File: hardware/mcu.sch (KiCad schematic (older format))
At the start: 57 parts, among them P3 CONN_01X09, P4 CONN_02X05_JTAG, P5 CONN_01X03_UART, P6 CONN_01X03_CAN, P7 CONN_01X05_ENCODER, SW2 SW_PUSH, U13 TM4C1294KCPDT, U14 74LVCH2T45, U15 SN65HVD231D, Y1 NX5032GA

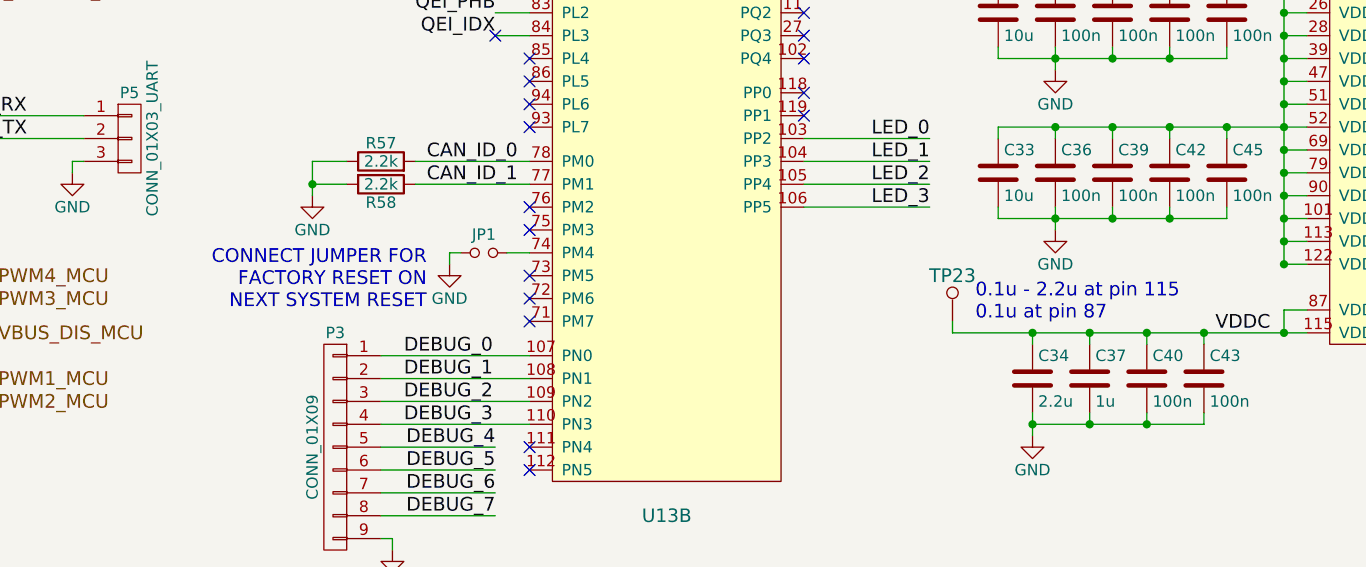
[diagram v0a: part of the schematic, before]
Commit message: tweaks, testpoints, decluttering
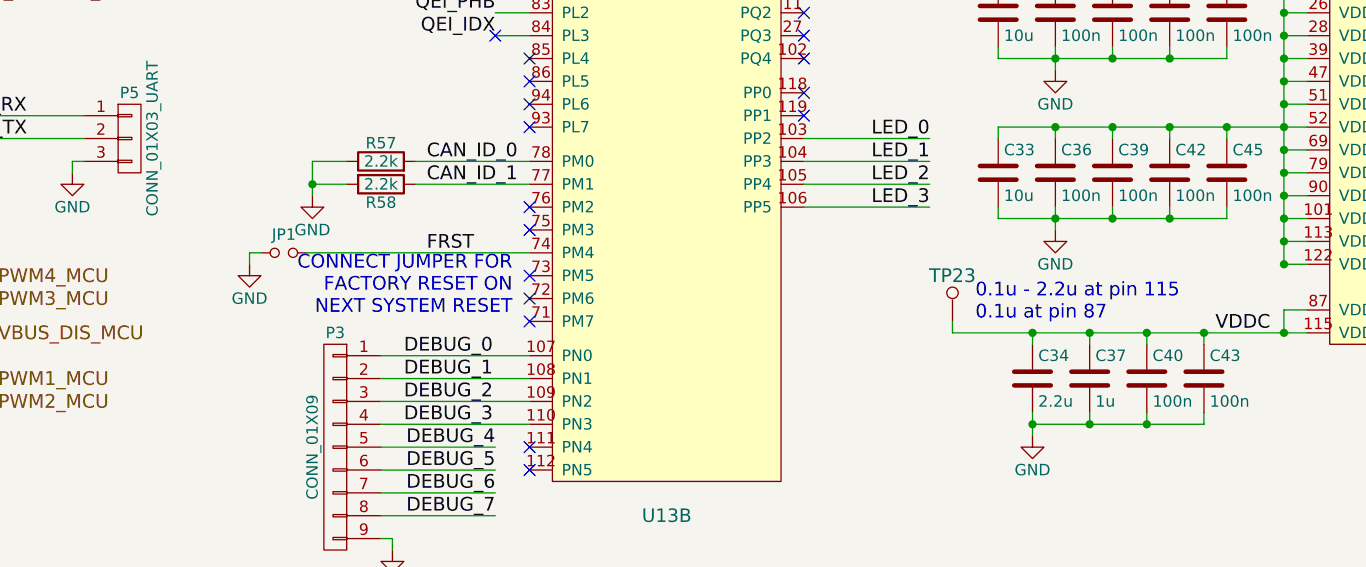
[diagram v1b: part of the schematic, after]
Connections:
- net FRST: now reaches JP1.1, U13.74 (PM4)
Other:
- moved on the sheet: JP1
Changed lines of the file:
@@
 L Jumper_NO_Small JP1
 U 1 1 59C1D74D
-P 5850 2300
-F 0 "JP1" H 5850 2380 50  0000 C CNN
-F 1 "Jumper_NO_Small" H 5860 2240 50  0001 C CNN
-F 2 "Pin_Headers:Pin_Header_Straight_1x02" H 5850 2300 50  0001 C CNN
-F 3 "" H 5850 2300 50  0000 C CNN
-	1    5850 2300
+P 4975 2300
+F 0 "JP1" H 4975 2380 50  0000 C CNN
+F 1 "Jumper_NO_Small" H 4985 2240 50  0001 C CNN
+F 2 "Pin_Headers:Pin_Header_Straight_1x02" H 4975 2300 50  0001 C CNN
+F 3 "" H 4975 2300 50  0000 C CNN
+	1    4975 2300
 	-1   0    0    -1
 $EndComp
@@
 L GND #PWR091
 U 1 1 59C1E162
-P 5700 2350
-F 0 "#PWR091" H 5700 2100 50  0001 C CNN
-F 1 "GND" H 5700 2200 50  0000 C CNN
-F 2 "" H 5700 2350 50  0000 C CNN
-F 3 "" H 5700 2350 50  0000 C CNN
-	1    5700 2350
+P 4825 2350
+F 0 "#PWR091" H 4825 2100 50  0001 C CNN
+F 1 "GND" H 4825 2200 50  0000 C CNN
+F 2 "" H 4825 2350 50  0000 C CNN
+F 3 "" H 4825 2350 50  0000 C CNN
+	1    4825 2350
 	-1   0    0    -1
 $EndComp
-Text Notes 5600 2550 2    60   ~ 0
+Text Notes 5975 2575 2    60   ~ 0
 CONNECT JUMPER FOR\nFACTORY RESET ON\nNEXT SYSTEM RESET
 $Comp
@@
 	8250 2700 8250 2650
 Wire Wire Line
-	8500 2700 8500 2650
+	8500 2650 8500 2700
 Connection ~ 8500 2650
 Wire Wire Line
-	8750 2700 8750 2650
+	8750 2650 8750 2700
 Connection ~ 8750 2650
 Wire Wire Line
@@
 Connection ~ 8500 3050
 Wire Wire Line
-	9000 2700 9000 2650
+	9000 2650 9000 2700
 Connection ~ 9000 2650
 Wire Wire Line
@@
 	3050 4800 3050 4700
 Wire Wire Line
-	6050 2300 5950 2300
-Wire Wire Line
-	5750 2300 5700 2300
-Wire Wire Line
-	5700 2300 5700 2350
+	6050 2300 5075 2300
+Wire Wire Line
+	4875 2300 4825 2300
+Wire Wire Line
+	4825 2300 4825 2350
 Wire Wire Line
 	4550 5150 4550 5250
@@
 Wire Wire Line
 	7900 2650 9450 2650
+Text Label 5600 2300 0    60   ~ 0
+FRST
 $EndSCHEMATC
